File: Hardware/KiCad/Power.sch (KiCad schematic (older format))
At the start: 28 parts, among them J19 POWER_JACKPTH, Q4 FDN340P, Q5 FDN340P, SW1 SW_SPDT, U2 LM358, U3 AMS1117-3.3, U8 MP2307SO

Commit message: preparando archivos
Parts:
- C10, C11, C15, C16, C22, C23, C24, C8: symbol C_Small -> Grape:C_Small
- C7, C9: symbol CP1_Small -> Grape:CP1_Small
- D1: symbol MBRA140 -> Grape:MBRA140
- J19: symbol POWER_JACKPTH -> Grape:POWER_JACKPTH
- L1, L2: symbol L_Small -> Grape:L_Small
- Q4, Q5: symbol MOSFET-PCHANNEL -> Grape:MOSFET-PCHANNEL
- R10, R11, R16, R17, R18, R20, R7, R9: symbol R_Small -> Grape:R_Small
- SW1: symbol SW_SPDT -> Grape:SW_SPDT
- U2: symbol LM358 -> Grape:LM358
- U3: symbol V_REG_LM1117SOT223 -> Grape:V_REG_LM1117SOT223
- U8: symbol MP2307SO -> Grape:MP2307SO
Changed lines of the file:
@@
-EESchema Schematic File Version 2
-LIBS:Grape
-EELAYER 25 0
+EESchema Schematic File Version 4
+LIBS:Grape-cache
+EELAYER 26 0
 EELAYER END
 $Descr A4 11693 8268
@@
 $EndDescr
 $Comp
-L POWER_JACKPTH J19
+L Grape:POWER_JACKPTH J19
 U 1 1 5A5C9961
 P 2900 2550
@@
 $EndComp
 $Comp
-L MBRA140 D1
+L Grape:MBRA140 D1
 U 1 1 5A5C99D2
 P 3950 2250
@@
 $EndComp
 $Comp
-L SW_SPDT SW1
+L Grape:SW_SPDT SW1
 U 1 1 5A5C9A3B
 P 3450 2250
@@
 	3750 2250 3850 2250
 $Comp
-L GND #PWR077
+L Grape:GND #PWR077
 U 1 1 5A5C9A9A
 P 3150 2650
@@
 Connection ~ 3150 2450
 $Comp
-L MP2307SO U8
+L Grape:MP2307SO U8
 U 1 1 5A5BF038
 P 5900 2450
@@
 $EndComp
 $Comp
-L R_Small R9
+L Grape:R_Small R9
 U 1 1 5A5BF0D7
 P 6500 2950
@@
 $EndComp
 $Comp
-L C_Small C8
+L Grape:C_Small C8
 U 1 1 5A5BF0F6
 P 6750 2800
@@
 $EndComp
 $Comp
-L L_Small L1
+L Grape:L_Small L1
 U 1 1 5A5BF1D1
 P 6900 2250
@@
 $EndComp
 $Comp
-L L_Small L2
+L Grape:L_Small L2
 U 1 1 5A5BF248
 P 8600 2250
@@
 $EndComp
 $Comp
-L LM358 U2
+L Grape:LM358 U2
 U 1 1 5A5BF280
 P 4200 4750
@@
 $EndComp
 $Comp
-L LM358 U2
+L Grape:LM358 U2
 U 2 1 5A5BF2D1
 P 4800 5600
@@
 $EndComp
 $Comp
-L MOSFET-PCHANNEL Q5
+L Grape:MOSFET-PCHANNEL Q5
 U 1 1 5A5BF799
 P 6050 5250
@@
 $EndComp
 $Comp
-L V_REG_LM1117SOT223 U3
+L Grape:V_REG_LM1117SOT223 U3
 U 1 1 5A5BF9C1
 P 7700 4500
@@
 Connection ~ 4200 2250
 $Comp
-L CP1_Small C9
+L Grape:CP1_Small C9
 U 1 1 5A5C0005
 P 4200 2650
@@
 $EndComp
 $Comp
-L GND #PWR078
+L Grape:GND #PWR078
 U 1 1 5A5C01F7
 P 4400 2900
@@
 	4400 2850 4400 2900
 $Comp
-L C_Small C10
+L Grape:C_Small C10
 U 1 1 5A5C02FA
 P 4600 2650
@@
 	4600 2250 4600 2550
 $Comp
-L R_Small R11
+L Grape:R_Small R11
 U 1 1 5A5C056A
 P 4950 2250
@@
 VIN
 $Comp
-L C_Small C11
+L Grape:C_Small C11
 U 1 1 5A5C0F27
 P 5100 2700
@@
 $EndComp
 $Comp
-L GND #PWR079
+L Grape:GND #PWR079
 U 1 1 5A5C0F7F
 P 5100 2900
@@
 	5100 2450 5300 2450
 $Comp
-L GND #PWR080
+L Grape:GND #PWR080
 U 1 1 5A5C10E8
 P 5900 3150
@@
 Connection ~ 5900 3050
 $Comp
-L GND #PWR081
+L Grape:GND #PWR081
 U 1 1 5A5C1430
 P 6300 3150
@@
 	6750 2950 6750 2900
 $Comp
-L C_Small C16
+L Grape:C_Small C16
 U 1 1 5A5C1DE2
 P 6400 1800
@@
 Connection ~ 6700 2250
 $Comp
-L R_Small R7
+L Grape:R_Small R7
 U 1 1 5A5C225B
 P 7400 2400
@@
 $EndComp
 $Comp
-L R_Small R10
+L Grape:R_Small R10
 U 1 1 5A5C23A7
 P 7400 2700
@@
 $EndComp
 $Comp
-L GND #PWR082
+L Grape:GND #PWR082
 U 1 1 5A5C23FE
 P 7400 3150
@@
 Connection ~ 7400 2550
 $Comp
-L CP1_Small C7
+L Grape:CP1_Small C7
 U 1 1 5A5C273B
 P 8200 2500
@@
 $EndComp
 $Comp
-L C_Small C15
+L Grape:C_Small C15
 U 1 1 5A5C28C1
 P 7850 2500
@@
 $EndComp
 $Comp
-L GND #PWR083
+L Grape:GND #PWR083
 U 1 1 5A5C2B61
 P 8050 3150
@@
 VDD5
 $Comp
-L C_Small C22
+L Grape:C_Small C22
 U 1 1 5A5C6DC1
 P 3150 4850
@@
 $EndComp
 $Comp
-L R_Small R18
+L Grape:R_Small R18
 U 1 1 5A5C6FAB
 P 2700 4450
@@
 $EndComp
 $Comp
-L R_Small R17
+L Grape:R_Small R17
 U 1 1 5A5C7277
 P 2700 4850
@@
 $EndComp
 $Comp
-L GND #PWR084
+L Grape:GND #PWR084
 U 1 1 5A5C72FB
 P 2700 5100
@@
 Connection ~ 3150 4650
 $Comp
-L GND #PWR085
+L Grape:GND #PWR085
 U 1 1 5A5C7D92
 P 3150 5100
@@
 	3150 4950 3150 5100
 $Comp
-L +3.3V #PWR086
+L Grape:+3.3V #PWR086
 U 1 1 5A5C80BD
 P 3750 4250
@@
 Connection ~ 3550 4650
 $Comp
-L GND #PWR087
+L Grape:GND #PWR087
 U 1 1 5A5C8333
 P 4100 5100
@@
 	4100 5050 4100 5100
 $Comp
-L GND #PWR088
+L Grape:GND #PWR088
 U 1 1 5A5C859C
 P 4700 5950
@@
 $EndComp
 $Comp
-L +5V #PWR089
+L Grape:+5V #PWR089
 U 1 1 5A5C88D0
 P 4700 5200
@@
 	6450 5250 6450 5150
 $Comp
-L MOSFET-PCHANNEL Q4
+L Grape:MOSFET-PCHANNEL Q4
 U 1 1 5A5BF6D6
 P 5600 4400
@@
 	4500 4750 5600 4750
 $Comp
-L R_Small R20
+L Grape:R_Small R20
 U 1 1 5A5C9C0D
 P 4900 4550
@@
 Connection ~ 4900 4750
 $Comp
-L R_Small R16
+L Grape:R_Small R16
 U 1 1 5A5C9ECA
 P 5200 5400
@@
 	4900 4150 4900 4450
 $Comp
-L C_Small C23
+L Grape:C_Small C23
 U 1 1 5A5CA56B
 P 4500 4350
@@
 $EndComp
 $Comp
-L GND #PWR090
+L Grape:GND #PWR090
 U 1 1 5A5CA6CD
 P 4500 4500
@@
 Connection ~ 4900 4150
 $Comp
-L +5V #PWR091
+L Grape:+5V #PWR091
 U 1 1 5A5CA8D5
 P 4100 4050
@@
 	5600 4750 5600 4700
 $Comp
-L +5V #PWR092
+L Grape:+5V #PWR092
 U 1 1 5A5CB171
 P 5900 4350
@@
 	5900 4400 5900 4350
 $Comp
-L +5V #PWR093
+L Grape:+5V #PWR093
 U 1 1 5A5CB2A8
 P 6450 5150
@@
 	4700 5900 4700 5950
 $Comp
-L PWR_FLAG #FLG094
+L Grape:PWR_FLAG #FLG094
 U 1 1 5A5CCC7F
 P 6700 7350
@@
 $EndComp
 $Comp
-L PWR_FLAG #FLG095
+L Grape:PWR_FLAG #FLG095
 U 1 1 5A5CCD01
 P 6250 7350
@@
 $EndComp
 $Comp
-L PWR_FLAG #FLG096
+L Grape:PWR_FLAG #FLG096
 U 1 1 5A5CCF50
 P 5900 7000
@@
 $EndComp
 $Comp
-L GND #PWR097
+L Grape:GND #PWR097
 U 1 1 5A5CCFAF
 P 5900 7350
@@
 	5900 7350 5900 7000
 $Comp
-L +5V #PWR098
+L Grape:+5V #PWR098
 U 1 1 5A5CD193
 P 6250 7000
@@
 	6250 7000 6250 7350
 $Comp
-L +3.3V #PWR099
+L Grape:+3.3V #PWR099
 U 1 1 5A5CD3CC
 P 6700 7000
@@
 $EndComp
 $Comp
-L C_Small C24
+L Grape:C_Small C24
 U 1 1 5A5CD924
 P 8400 4700
@@
 $EndComp
 $Comp
-L +5V #PWR0100
+L Grape:+5V #PWR0100
 U 1 1 5A5CDF65
 P 7100 4350
@@
 	7100 4500 7400 4500
 $Comp
-L GND #PWR0101
+L Grape:GND #PWR0101
 U 1 1 5A5CE207
 P 7700 4900
@@
 	8000 4500 8500 4500
 $Comp
-L GND #PWR0102
+L Grape:GND #PWR0102
 U 1 1 5A5CE552
 P 8400 4900
@@
 Connection ~ 8400 4500
 $Comp
-L +3.3V #PWR0103
+L Grape:+3.3V #PWR0103
 U 1 1 5A5CEA4E
 P 8500 4400
@@
 $Bitmap
 Pos 10850 6250
-Scale 0,950000
+Scale 0.000000
 Data
 89 50 4E 47 0D 0A 1A 0A 00 00 00 0D 49 48 44 52 00 00 00 C1 00 00 00 8F 08 06 00 00 00 43 10 BF
@@
 $Bitmap
 Pos 7300 6700
-Scale 0,950000
+Scale 0.000000
 Data
 89 50 4E 47 0D 0A 1A 0A 00 00 00 0D 49 48 44 52 00 00 00 91 00 00 00 36 08 06 00 00 00 C7 C1 7B

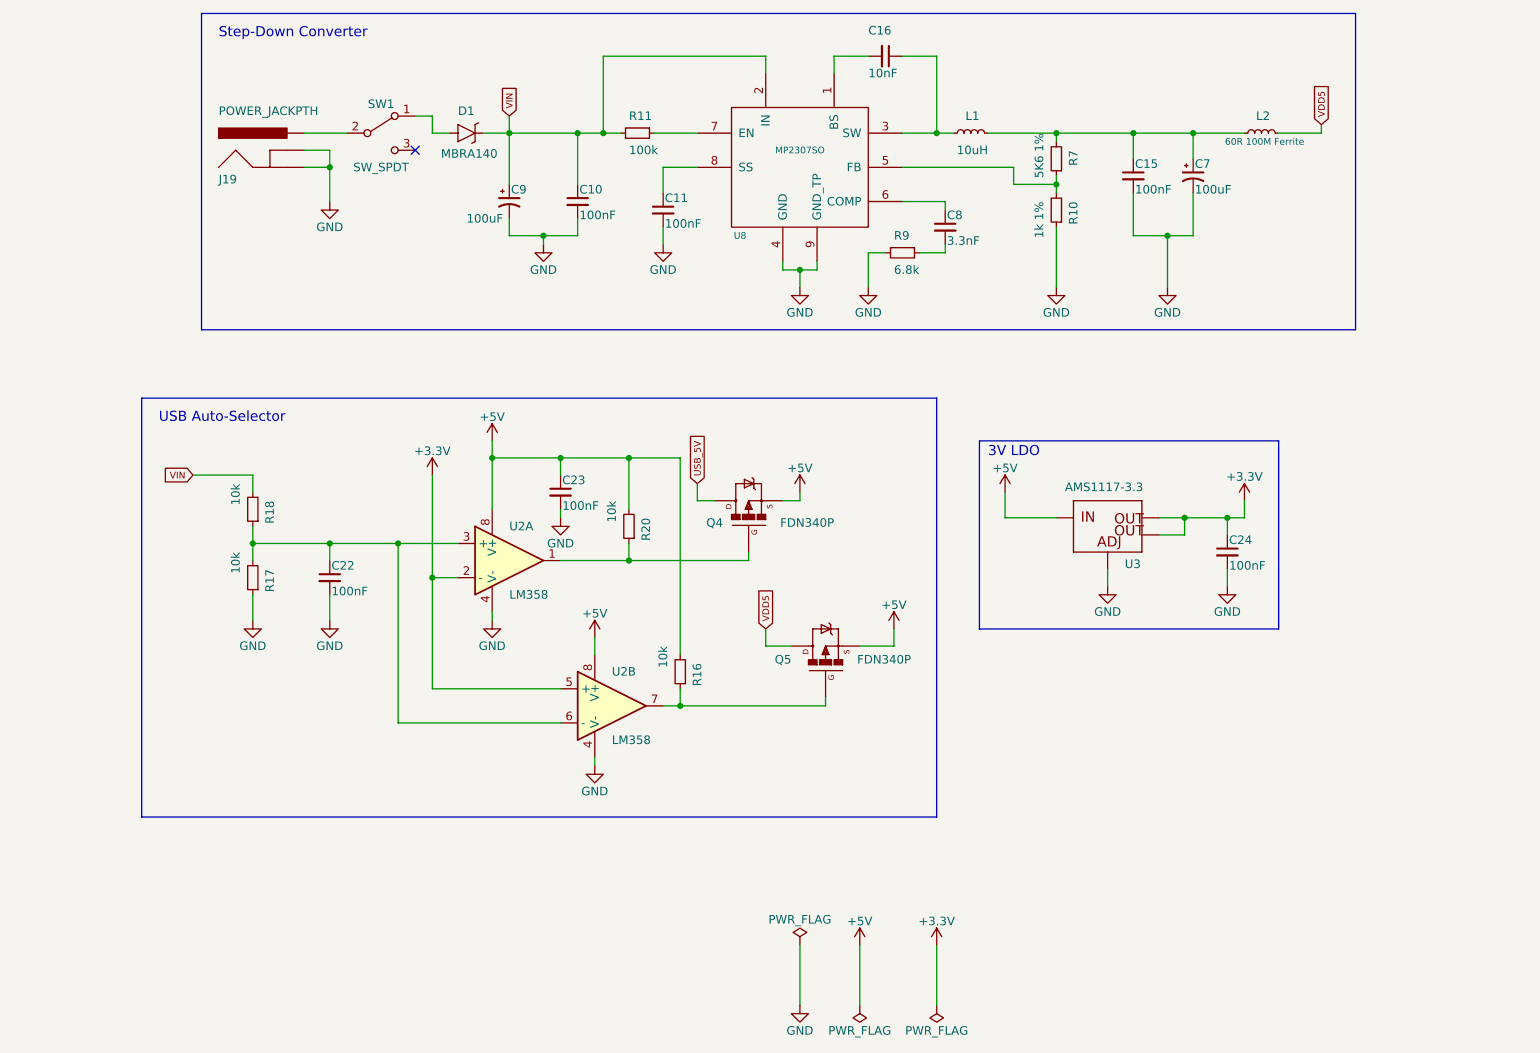
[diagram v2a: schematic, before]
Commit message: Esquema terminado
Falta comprobar
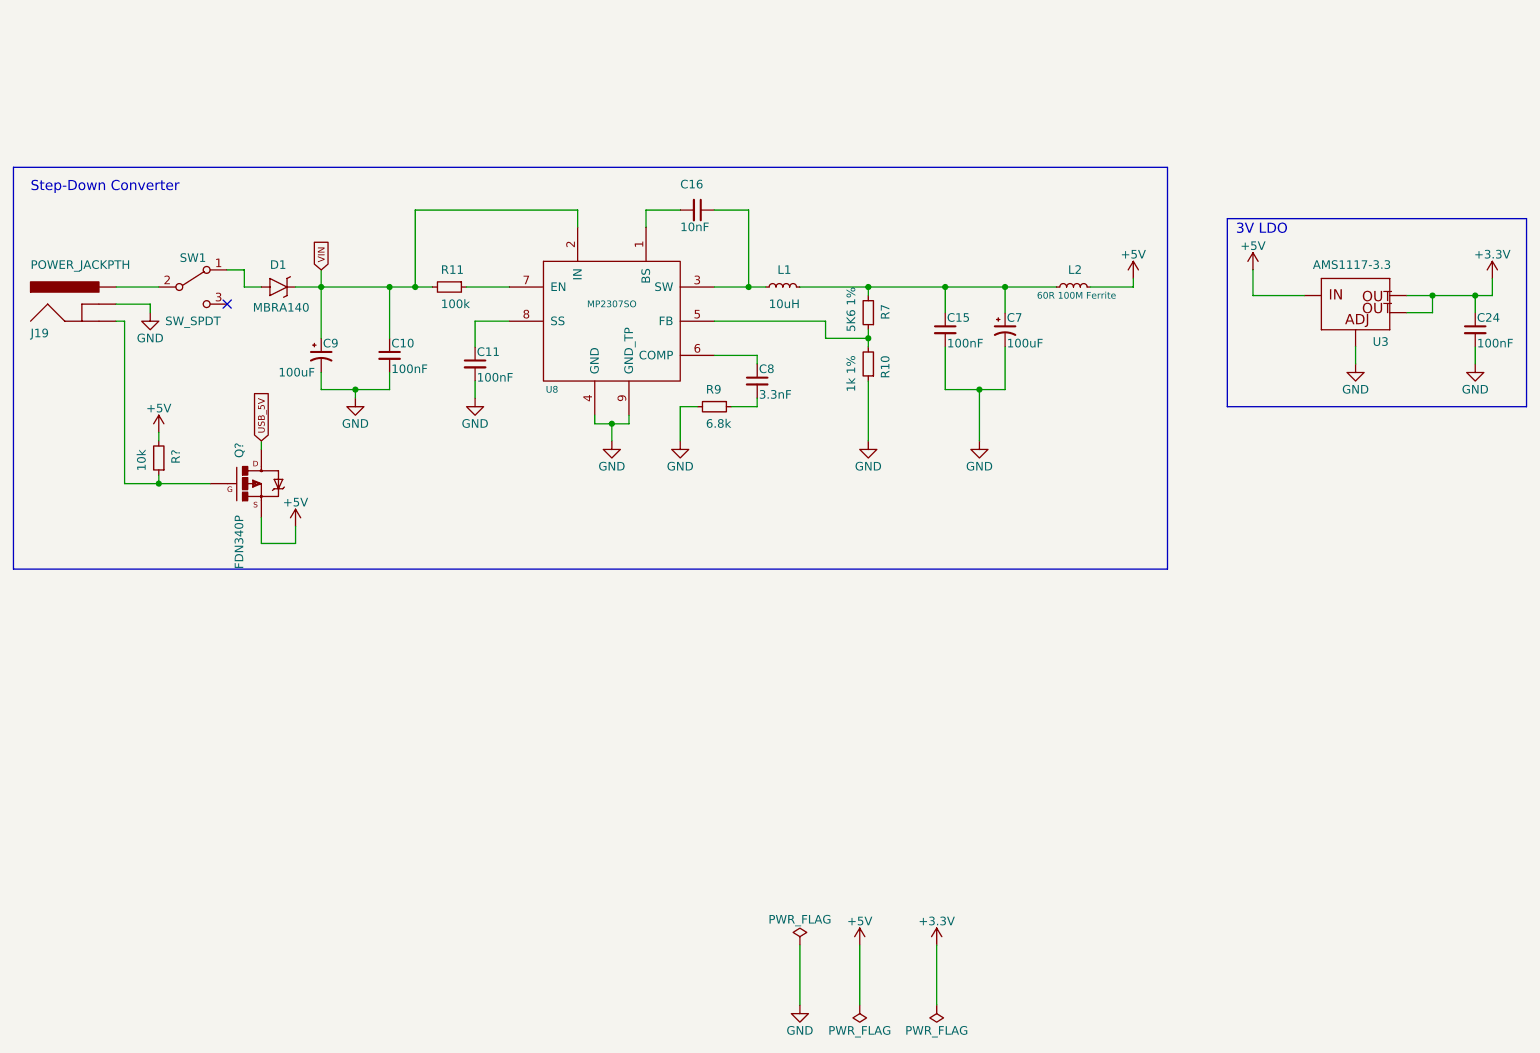
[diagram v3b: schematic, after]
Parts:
- removed C22, C23: 100nF, lib_sch:C_0805, symbol Grape:C_Small
- removed Q4, Q5: FDN340P, lib_sch:SOT-23, symbol Grape:MOSFET-PCHANNEL
- removed R16, R17, R18, R20: 10k, lib_sch:R_0805, symbol Grape:R_Small
- removed U2: LM358, lib_sch:SOIC-8_3.9x4.9mm_Pitch1.27mm, symbol Grape:LM358
- added Q?: FDN340P, lib_sch:SOT-23, symbol Grape:MOSFET-PCHANNEL
- added R?: 10k, lib_sch:R_0805, symbol Grape:R_Small
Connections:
- net VDD5 is gone; now on net +5V: L2.2
- net +5V: now also Q?.2 (S), R?.2
- net GND: no longer J19.3 (GND)
- net USB_5V: now also Q?.3 (D)
- new net: J19.3 (GND), Q?.1 (G), R?.1
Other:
- note removed: "USB Auto-Selector"
- moved on the sheet: C10, C11, C15, C16, C24, C7, C8, C9, D1, J19, L1, L2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
